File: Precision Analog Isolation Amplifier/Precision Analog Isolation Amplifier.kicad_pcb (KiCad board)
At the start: 2 copper layers, 59 parts, among them IC1 ADA4899-1YRDZ, J1 Conn_01x03, J2 Conn_01x03, J3 Conn_Coaxial, J4 Conn_Coaxial, Q1 ---, U1 HCNR201, U2 ADA4522, U4 ADA4522

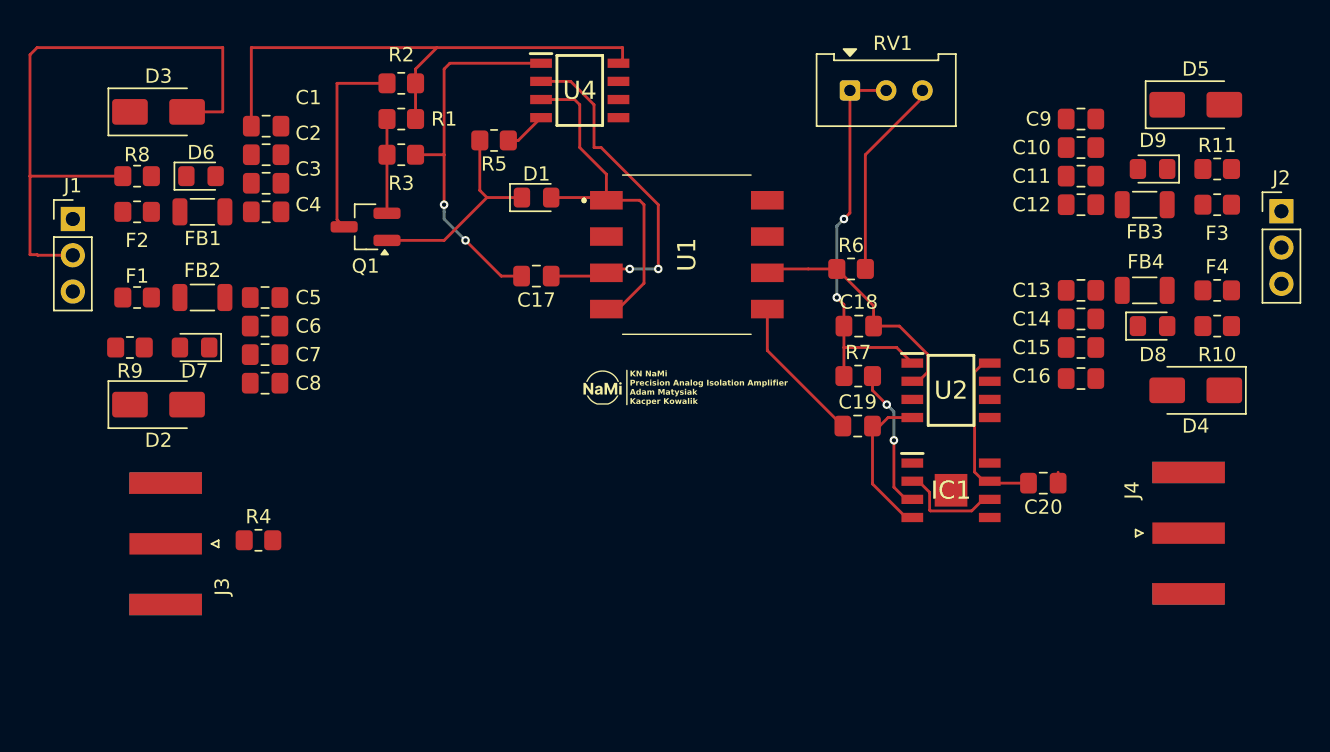
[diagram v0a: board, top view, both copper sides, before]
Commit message: Update PCB layout
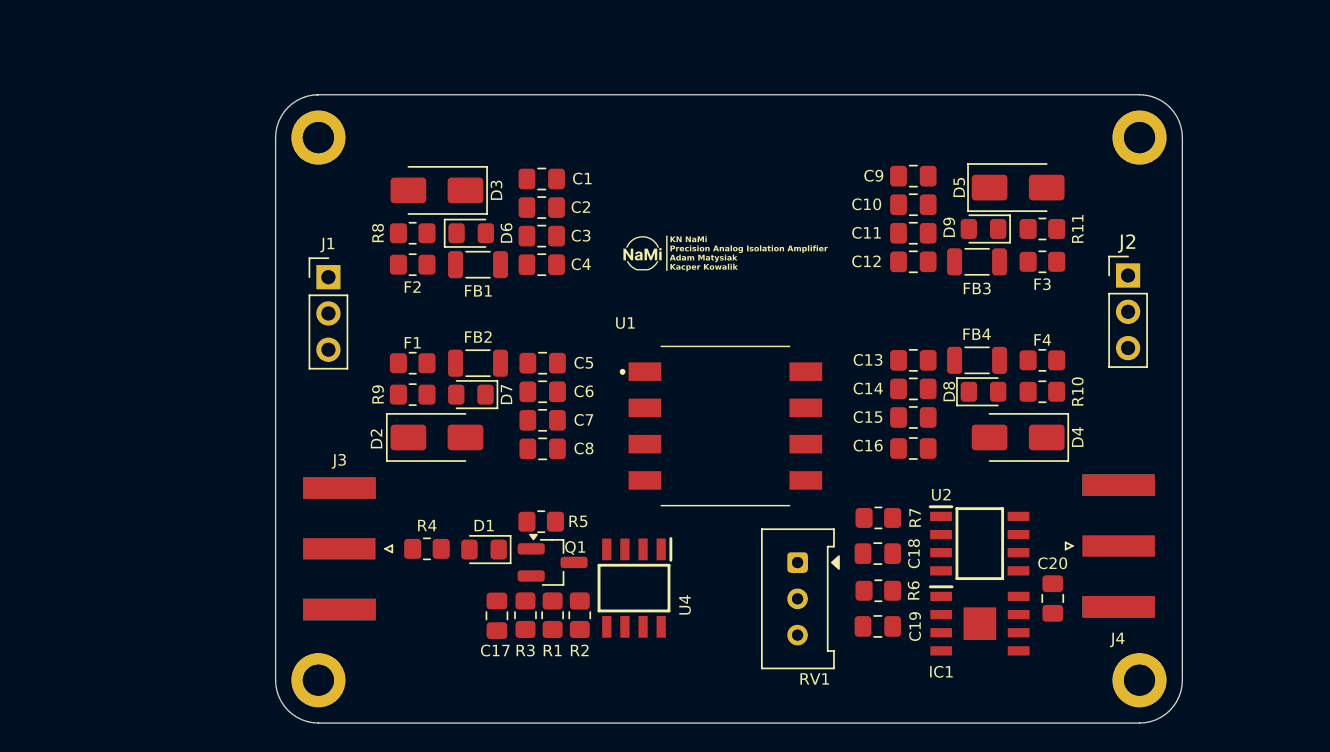
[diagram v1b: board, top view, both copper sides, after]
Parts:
- added REF**: MountingHole_2.2mm_M2_DIN965_Pad, MountingHole:MountingHole_2.2mm_M2_DIN965_Pad, F.Cu at (171.2, 117.3)
- added REF**: MountingHole_2.2mm_M2_DIN965_Pad, MountingHole:MountingHole_2.2mm_M2_DIN965_Pad, F.Cu at (171.2, 79.3)
- added REF**: MountingHole_2.2mm_M2_DIN965_Pad, MountingHole:MountingHole_2.2mm_M2_DIN965_Pad, F.Cu at (113.7, 79.3)
- added REF**: MountingHole_2.2mm_M2_DIN965_Pad, MountingHole:MountingHole_2.2mm_M2_DIN965_Pad, F.Cu at (113.7, 117.3)
- moved R2 39.3 mm to (132.0, 112.8), turned to 90 degrees
- moved R1 36.3 mm to (130.1, 112.8), turned to 90 degrees
- moved U4 35.1 mm to (135.8, 110.8), turned to -90 degrees
- moved R3 33.4 mm to (128.2, 112.8), turned to -90 degrees
- moved RV1 33.3 mm to (147.3, 109.1), turned to -90 degrees
- moved Q1 26.9 mm to (130.1, 109.0), turned to 0 degrees
- moved R5 26.9 mm to (129.3, 106.2), turned to 0 degrees
- moved D1 24.9 mm to (125.3, 108.2), turned to 180 degrees
- moved C17 23.9 mm to (126.2, 112.8), turned to -90 degrees
- moved R6 22.6 mm to (152.9, 111.0)
- moved D3 20.3 mm to (122.0, 83.0), turned to 180 degrees
- moved R9 20.1 mm to (120.3, 97.3)
- moved C5 20.0 mm to (129.4, 95.1)
- moved C6 20.0 mm to (129.4, 97.1)
- moved C7 20.0 mm to (129.4, 99.1)
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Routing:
- net GND1: track 70.1 -> 0.00 mm
- net VCC1 +15V: track 38.3 -> 0.00 mm
- net Vsep_out: track 28.4 -> 0.00 mm, vias 2 -> 0
- net Net-(C17-Pad2): track 26.5 -> 0.00 mm, vias 2 -> 0
- net Net-(U1B-K): track 25.8 -> 0.00 mm, vias 2 -> 0
- net Net-(U1C-K): track 17.2 -> 0.00 mm
- net Net-(D1-K): track 14.9 -> 0.00 mm
- net Net-(R6-Pad2): track 14.2 -> 0.00 mm
- net Net-(Q1-E): track 13.8 -> 0.00 mm
- net GND2: track 13.1 -> 0.00 mm
- net VCC2 +15V: track 12.4 -> 0.00 mm
- net VEE2 -15V: track 10.9 -> 0.00 mm
- net Net-(IC1-+IN): track 10.0 -> 0.00 mm, vias 2 -> 0
- net Vout: track 7.35 -> 0.00 mm
- net Net-(Q1-B): track 6.60 -> 0.00 mm
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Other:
- board outline added: 63.5 x 44 mm
